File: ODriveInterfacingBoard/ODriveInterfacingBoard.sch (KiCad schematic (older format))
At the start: 30 parts, among them U1 ODrive

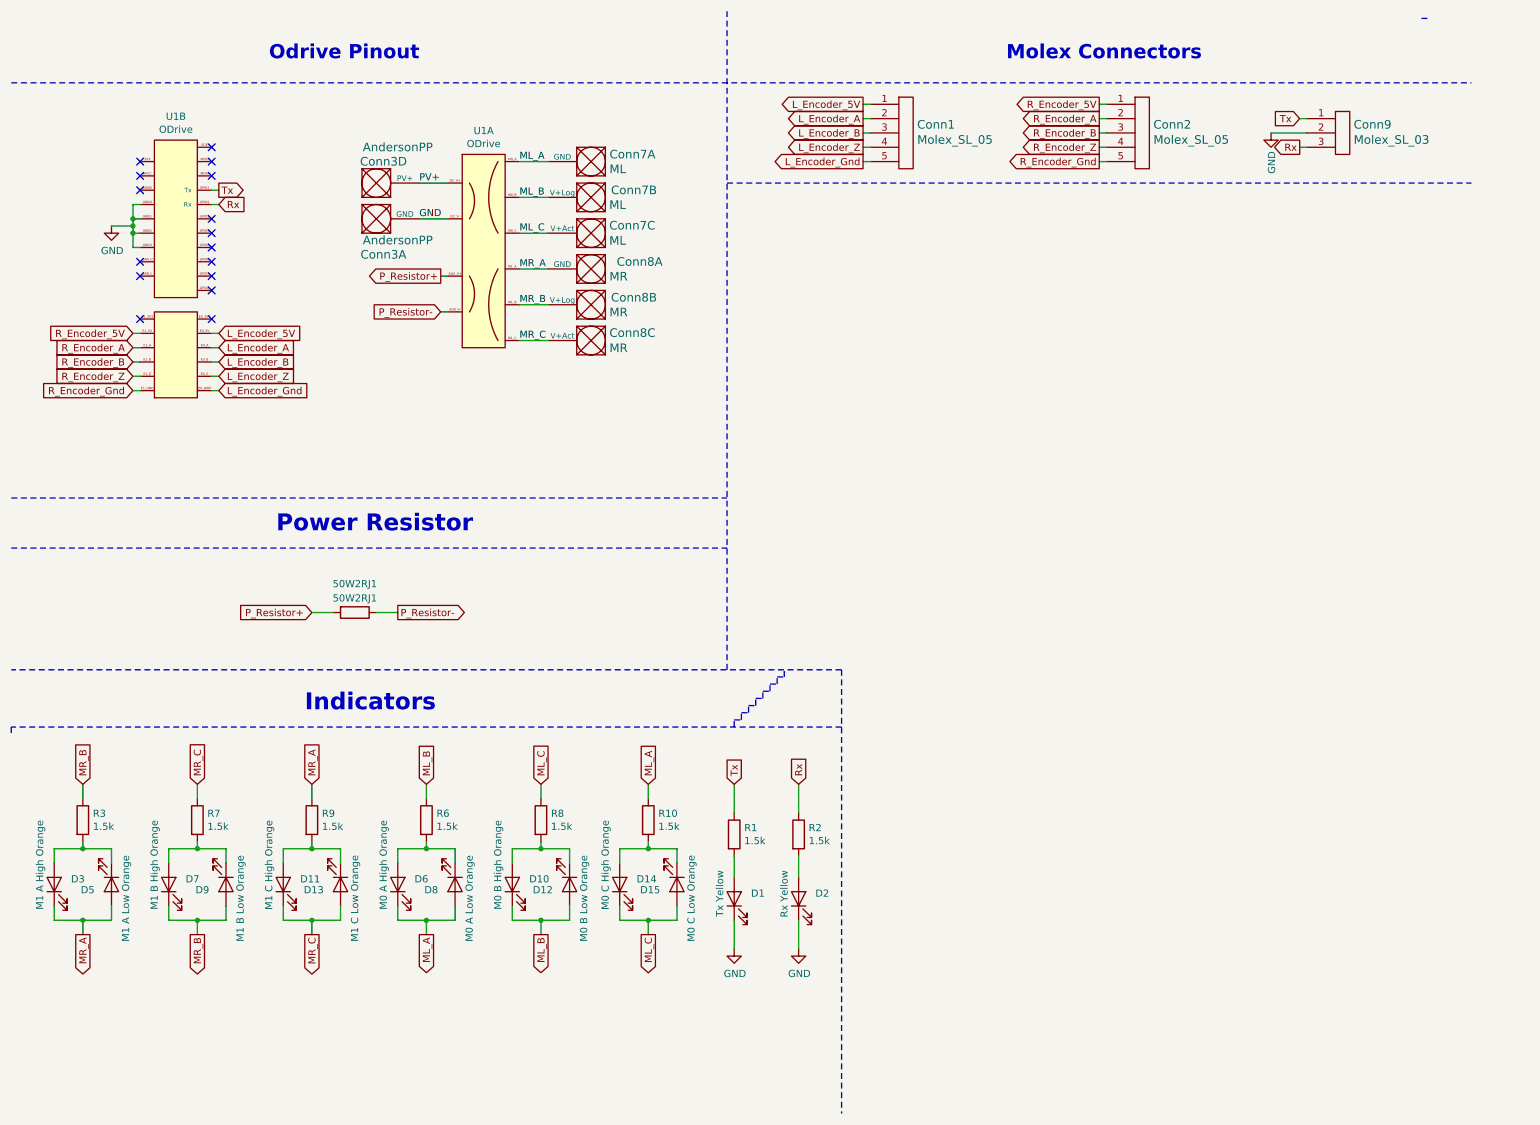
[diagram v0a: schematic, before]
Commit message: Just need silks and vias, babam
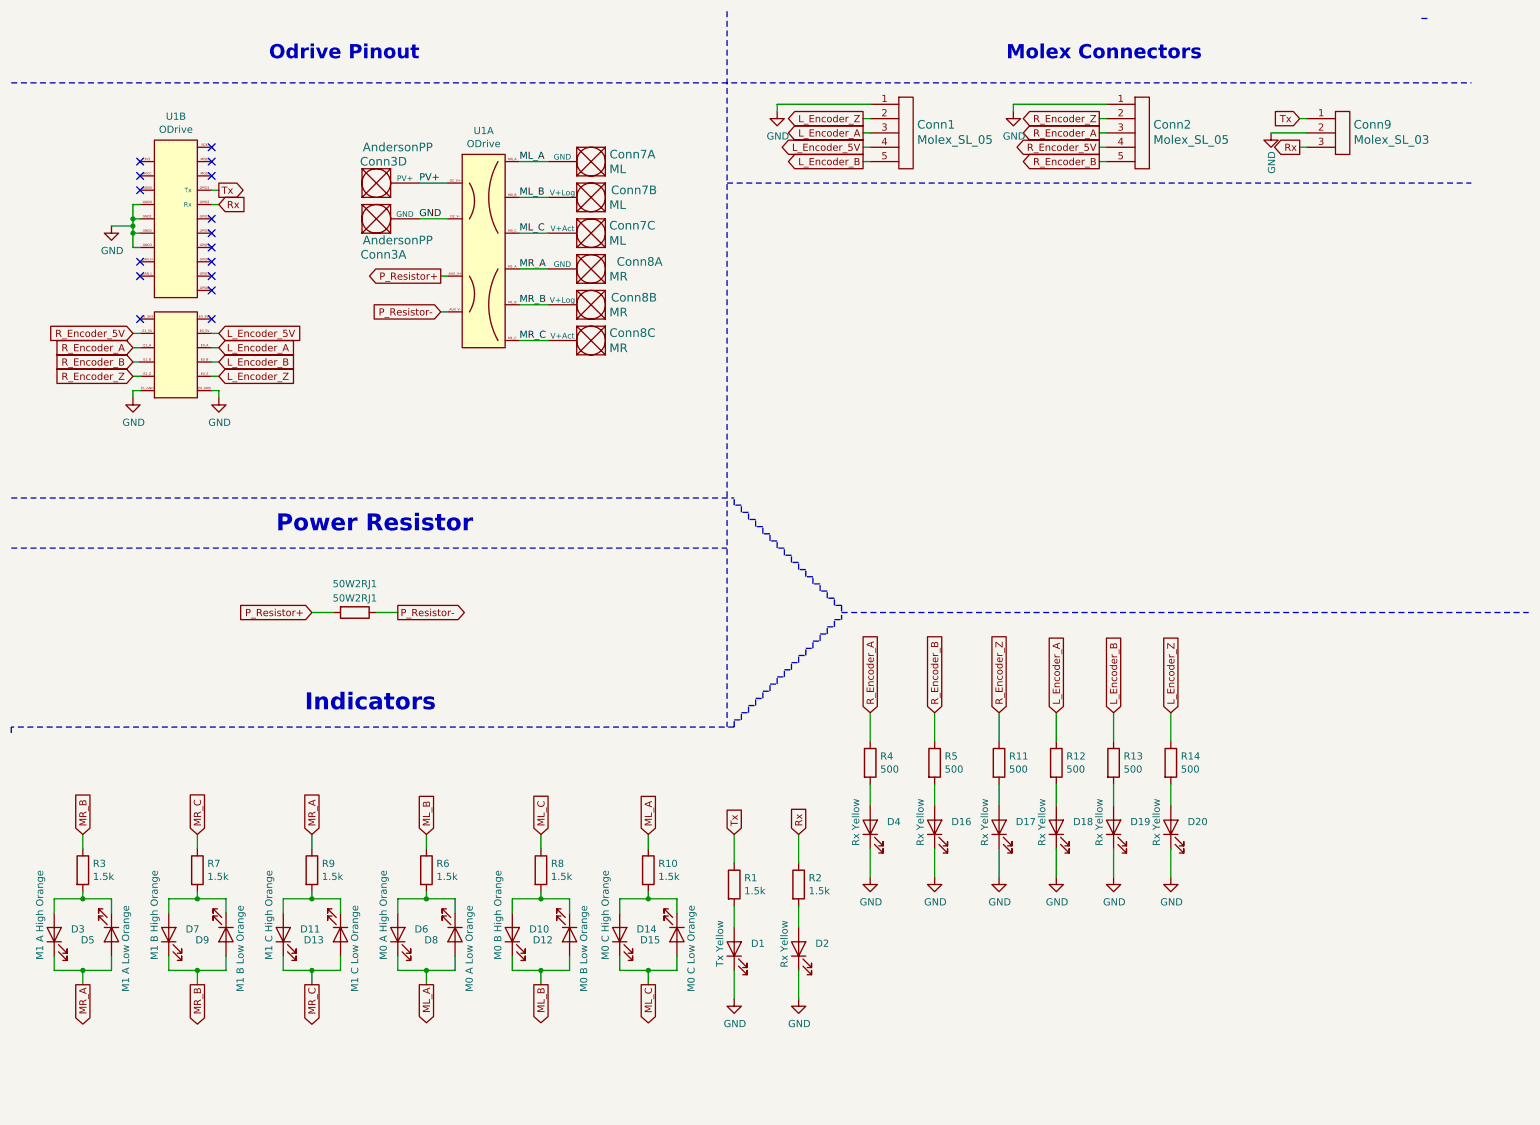
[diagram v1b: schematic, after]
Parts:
- added D16, D17, D18, D19, D20, D4: Rx Yellow, LED_SMD:LED_0603_1608Metric_Pad1.05x0.95mm_HandSolder, symbol ODriveInterfacingBoard-rescue:LED-Device
- added R11, R12, R13, R14, R4, R5: 500, Resistor_SMD:R_0603_1608Metric_Pad1.05x0.95mm_HandSolder, symbol ODriveInterfacingBoard-rescue:R-Device
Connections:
- net GND: now also Conn1.1, Conn2.1, U1.E0_GND, U1.E1_GND, D16.1 (K), D17.1 (K), D18.1 (K), D19.1 (K), D20.1 (K), D4.1 (K)
- net L_Encoder_5V: now also Conn1.4; no longer Conn1.1
- net L_Encoder_A: now also Conn1.3, R12.1; no longer Conn1.2
- net L_Encoder_B: now also Conn1.5, R13.1; no longer Conn1.3
- net L_Encoder_Z: now also Conn1.2, R14.1; no longer Conn1.4
- net R_Encoder_5V: now also Conn2.4; no longer Conn2.1
- net R_Encoder_A: now also Conn2.3, R4.1; no longer Conn2.2
- net R_Encoder_B: now also Conn2.5, R5.1; no longer Conn2.3
- net R_Encoder_Z: now also Conn2.2, R11.1; no longer Conn2.4
- removed net L_Encoder_Gnd: Conn1.5, U1.E0_GND
- removed net R_Encoder_Gnd: Conn2.5, U1.E1_GND
- new net: D4.2 (A), R4.2
- new net: D16.2 (A), R5.2
- new net: D17.2 (A), R11.2
- new net: D18.2 (A), R12.2
- new net: D19.2 (A), R13.2
- new net: D20.2 (A), R14.2
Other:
- moved on the sheet: D1, D10, D11, D12, D13, D14, D15, D2, D3, D5, D6, D7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
